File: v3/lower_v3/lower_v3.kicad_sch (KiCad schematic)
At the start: 5 parts, among them J1 Conn_01x09_MountingPin, J2 Conn_01x09_MountingPin, J4 Conn_01x02_Male, U1 ESP32-DEVKIT-V1

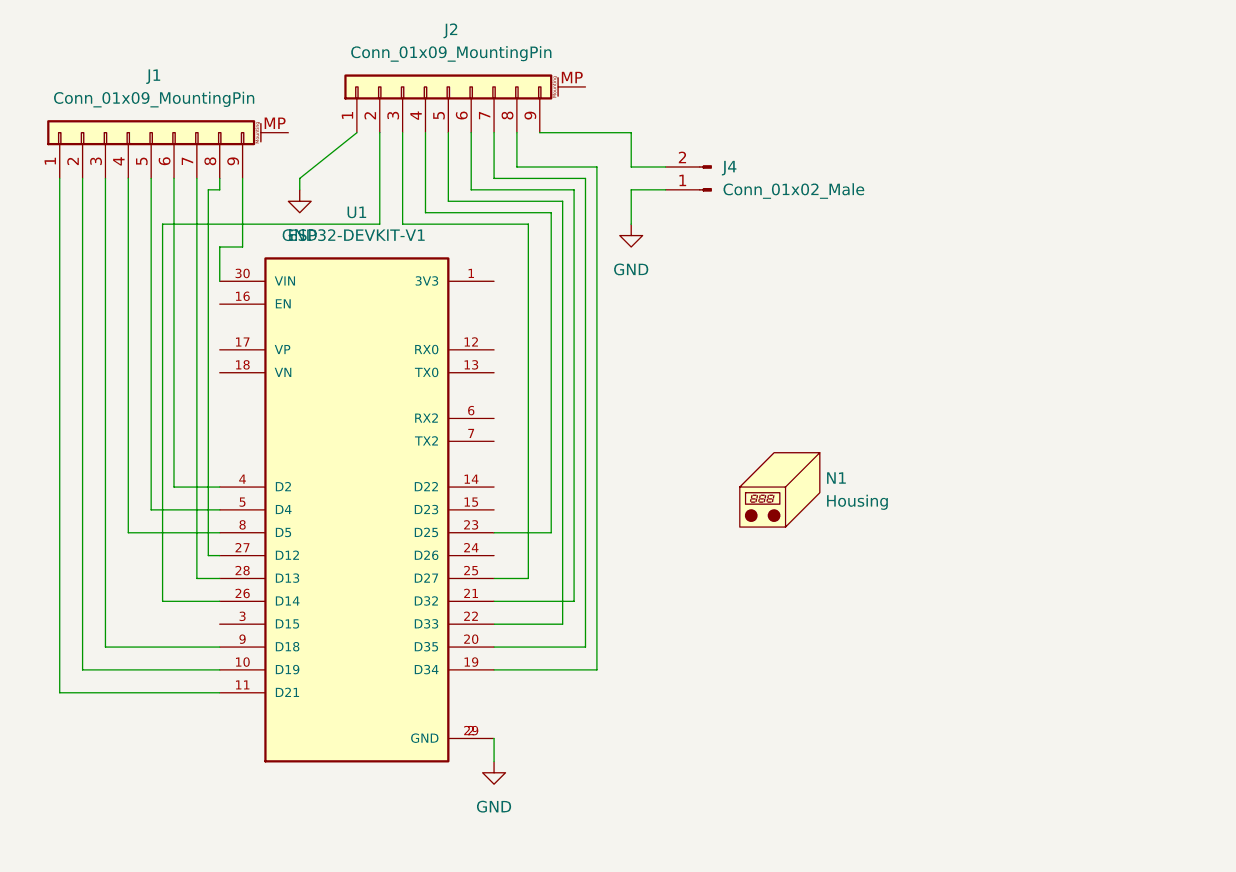
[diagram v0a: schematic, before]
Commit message: Complete Toast PCB
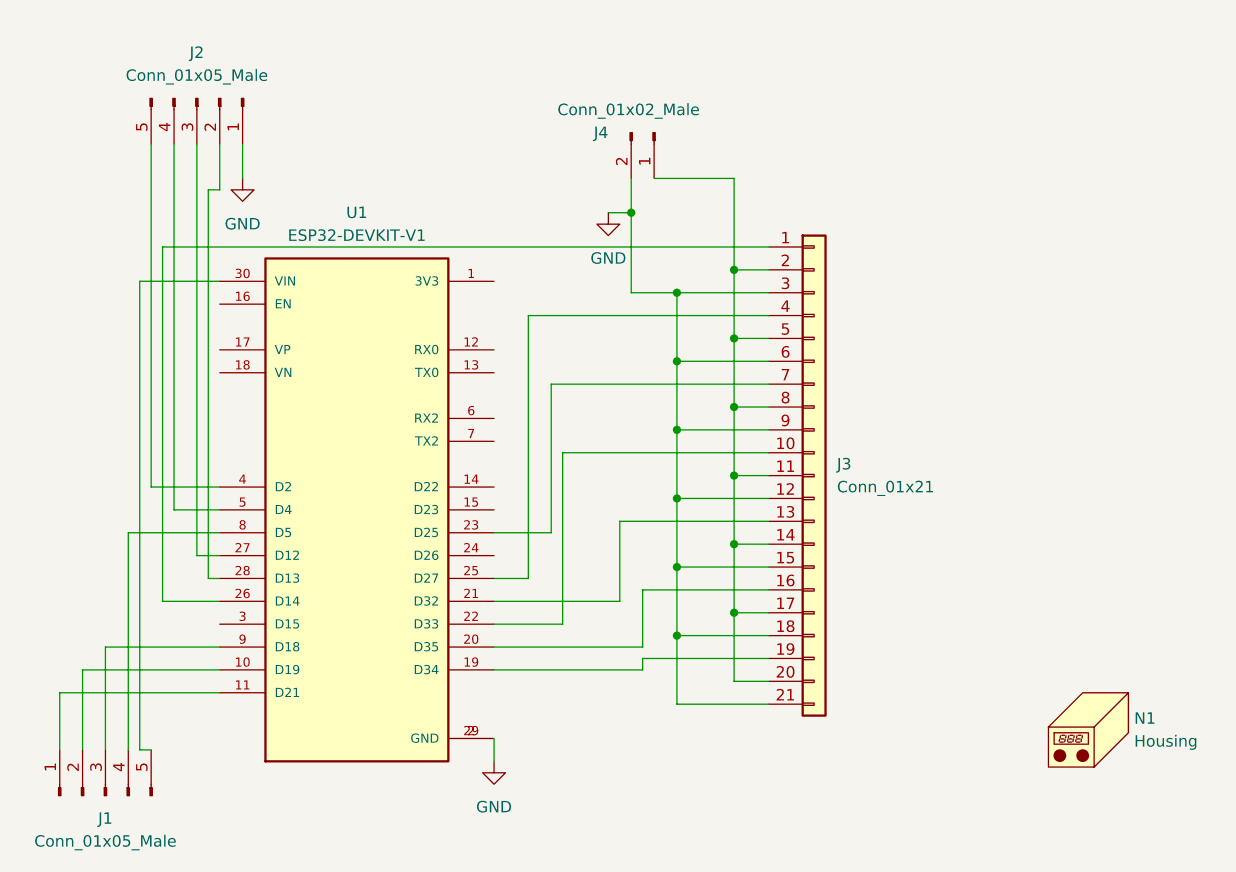
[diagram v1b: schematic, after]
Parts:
- removed J1, J2: Conn_01x09_MountingPin, Connector_PinSocket_2.54mm:PinSocket_1x09_P2.54mm_Vertical, symbol Connector_Generic_MountingPin:Conn_01x09_MountingPin
- added J1, J2: Conn_01x05_Male, Connector_PinHeader_2.54mm:PinHeader_1x05_P2.54mm_Vertical, symbol Connector:Conn_01x05_Male
- added J3: Conn_01x21, Connector_PinHeader_2.54mm:PinHeader_1x21_P2.54mm_Horizontal, symbol Connector_Generic:Conn_01x21
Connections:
- net GND: now also J4.2 (Pin_2), J2.1 (Pin_1), J3.12 (Pin_12), J3.15 (Pin_15), J3.18 (Pin_18), J3.21 (Pin_21), J3.3 (Pin_3), J3.6 (Pin_6), J3.9 (Pin_9); no longer J4.1 (Pin_1)
- net at U1.11 (D21): now also J1.1 (Pin_1)
- net at U1.10 (D19): now also J1.2 (Pin_2)
- net at U1.9 (D18): now also J1.3 (Pin_3)
- net at U1.8 (D5): now also J1.4 (Pin_4)
- net at U1.5 (D4): now also J2.4 (Pin_4)
- net at U1.4 (D2): now also J2.5 (Pin_5)
- net at U1.28 (D13): now also J2.2 (Pin_2)
- net at U1.27 (D12): now also J2.3 (Pin_3)
- net at U1.30 (VIN): now also J1.5 (Pin_5)
- net at U1.19 (D34): now also J3.19 (Pin_19)
- net at U1.20 (D35): now also J3.16 (Pin_16)
- net at U1.21 (D32): now also J3.13 (Pin_13)
- net at U1.22 (D33): now also J3.10 (Pin_10)
- net at U1.23 (D25): now also J3.7 (Pin_7)
- net at U1.25 (D27): now also J3.4 (Pin_4)
- net at U1.26 (D14): now also J3.1 (Pin_1)
- new net: J3.11 (Pin_11), J3.14 (Pin_14), J3.17 (Pin_17), J3.2 (Pin_2), J3.20 (Pin_20), J3.5 (Pin_5), J3.8 (Pin_8), J4.1 (Pin_1)
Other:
- moved on the sheet: J4, N1
